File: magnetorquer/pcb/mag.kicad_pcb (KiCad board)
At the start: 2 copper layers, 19 parts, among them J1 Conn_01x02, J2 Conn_01x02, U1 L293

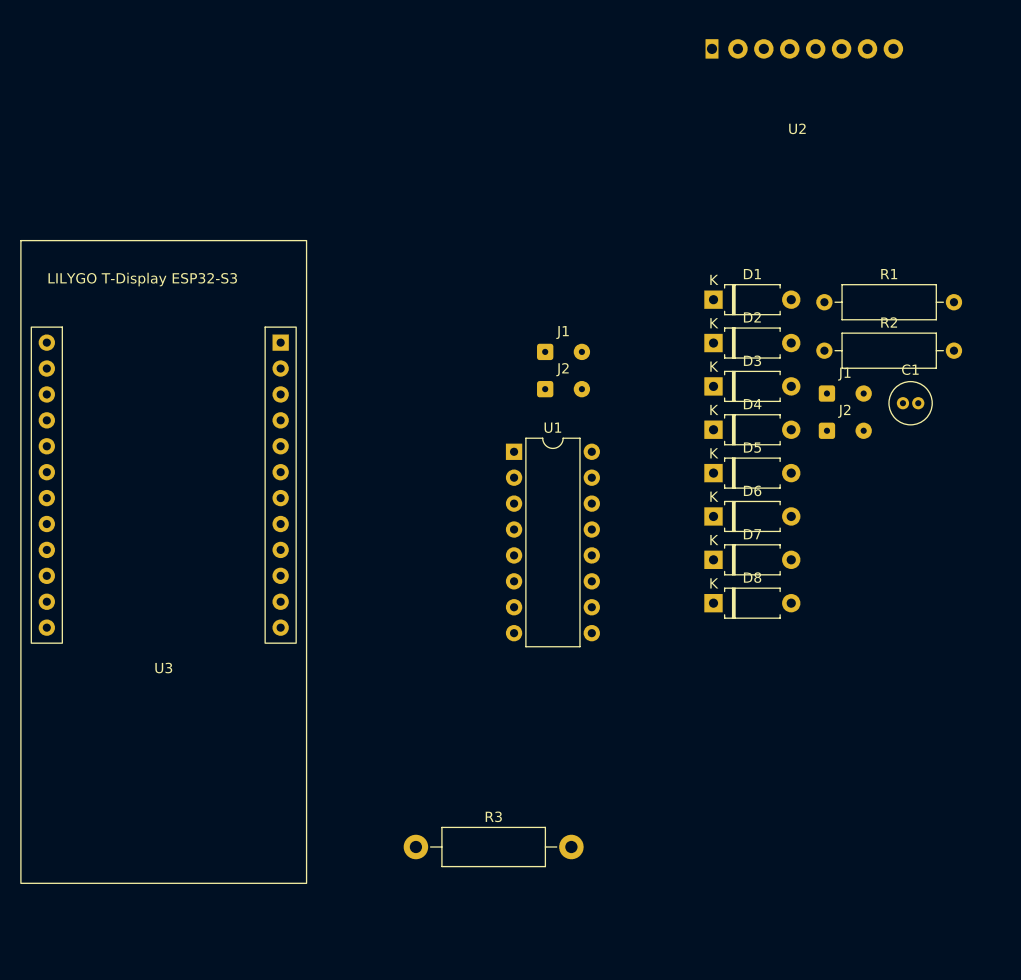
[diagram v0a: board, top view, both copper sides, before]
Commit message: feat: upload all changes for sch
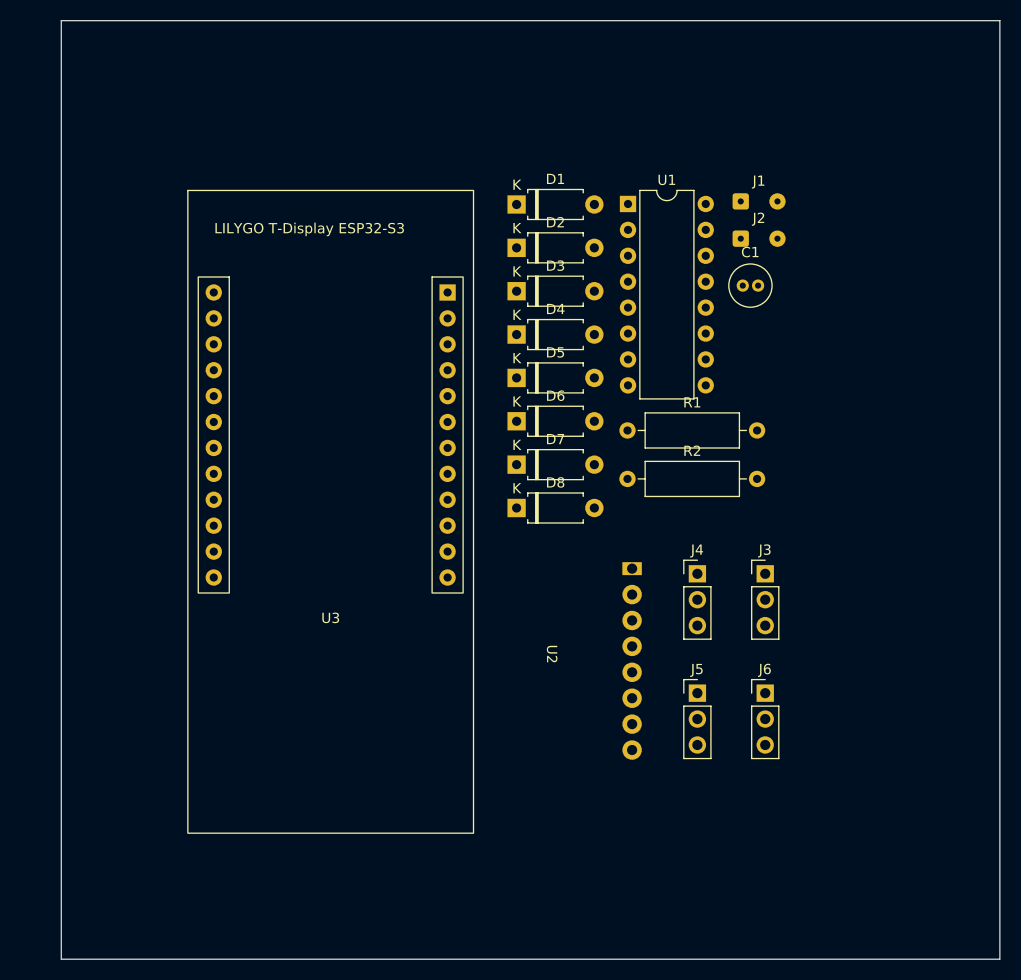
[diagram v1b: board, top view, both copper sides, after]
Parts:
- removed the J1 at (124.9, 83.0)
- removed the J1 at (152.6, 87.0)
- removed the J2 at (124.9, 86.6)
- removed the J2 at (152.6, 90.7)
- removed R3: R, Resistor_THT:R_Axial_DIN0411_L9.9mm_D3.6mm_P15.24mm_Horizontal
- added J1: Conn_01x02, Connector_Wire:SolderWire-0.1sqmm_1x02_P3.6mm_D0.4mm_OD1mm, F.Cu at (144.1, 68.2)
- added J2: Conn_01x02, Connector_Wire:SolderWire-0.1sqmm_1x02_P3.6mm_D0.4mm_OD1mm, F.Cu at (144.1, 71.9)
- added J3: Conn_01x03, Connector_PinHeader_2.54mm:PinHeader_1x03_P2.54mm_Vertical, F.Cu at (146.5, 104.7)
- added J4: Conn_01x03, Connector_PinHeader_2.54mm:PinHeader_1x03_P2.54mm_Vertical, F.Cu at (139.8, 104.7)
- added J5: Conn_01x03, Connector_PinHeader_2.54mm:PinHeader_1x03_P2.54mm_Vertical, F.Cu at (139.8, 116.4)
- added J6: Conn_01x03, Connector_PinHeader_2.54mm:PinHeader_1x03_P2.54mm_Vertical, F.Cu at (146.5, 116.4)
- moved U2 58.1 mm to (128.1, 112.6), turned to 0 degrees
- moved U1 26.7 mm to (133.1, 68.5)
- moved R1 23.0 mm to (133.0, 90.7)
- moved R2 23.0 mm to (133.0, 95.4)
- moved D1 21.4 mm to (122.1, 68.5)
- moved D2 21.4 mm to (122.1, 72.8)
- moved D3 21.4 mm to (122.1, 77.0)
- moved D4 21.4 mm to (122.1, 81.3)
- moved D5 21.4 mm to (122.1, 85.5)
- moved D6 21.4 mm to (122.1, 89.8)
- moved D7 21.4 mm to (122.1, 94.0)
- moved D8 21.4 mm to (122.1, 98.3)
- moved C1 19.5 mm to (144.3, 76.5)
- moved U3 17.1 mm to (103.9, 67.1)
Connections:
- net /ESP32/LDR_2 renamed /ESP32/LDR_Back
- net /ESP32/LDR_3 renamed /ESP32/LDR_Left
- net /ESP32/LDR_4 renamed /ESP32/LDR_Right
- U2 pad 4: /MPU-9255/SCL -> /ESP32/SCL
- U2 pad 5: /MPU-9255/SDA -> /ESP32/SDA
- U3 pad 17: /ESP32/MagI2C -> /ESP32/SDA
- U3 pad 18: /ESP32/MagI2C -> /ESP32/SCL
- U3 pad 2: /ESP32/LDR_1 -> /ESP32/LDR_Forward
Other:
- board outline added: 92 x 92 mm
